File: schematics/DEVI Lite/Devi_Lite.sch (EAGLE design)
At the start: 96 parts

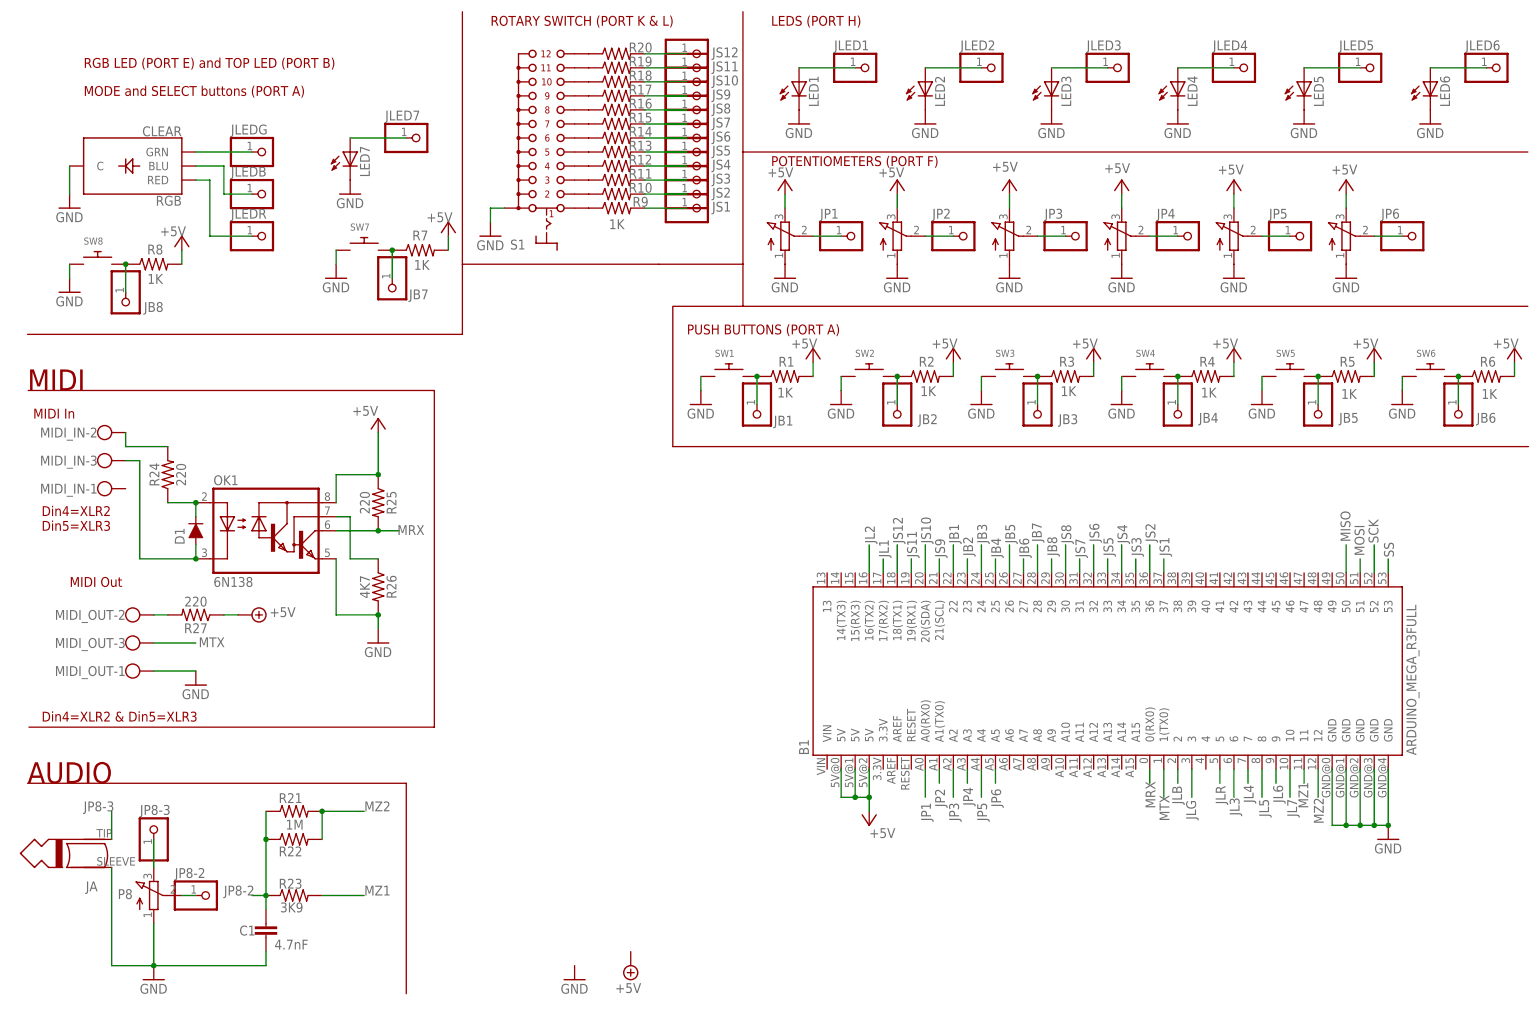
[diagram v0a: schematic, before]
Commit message: latest
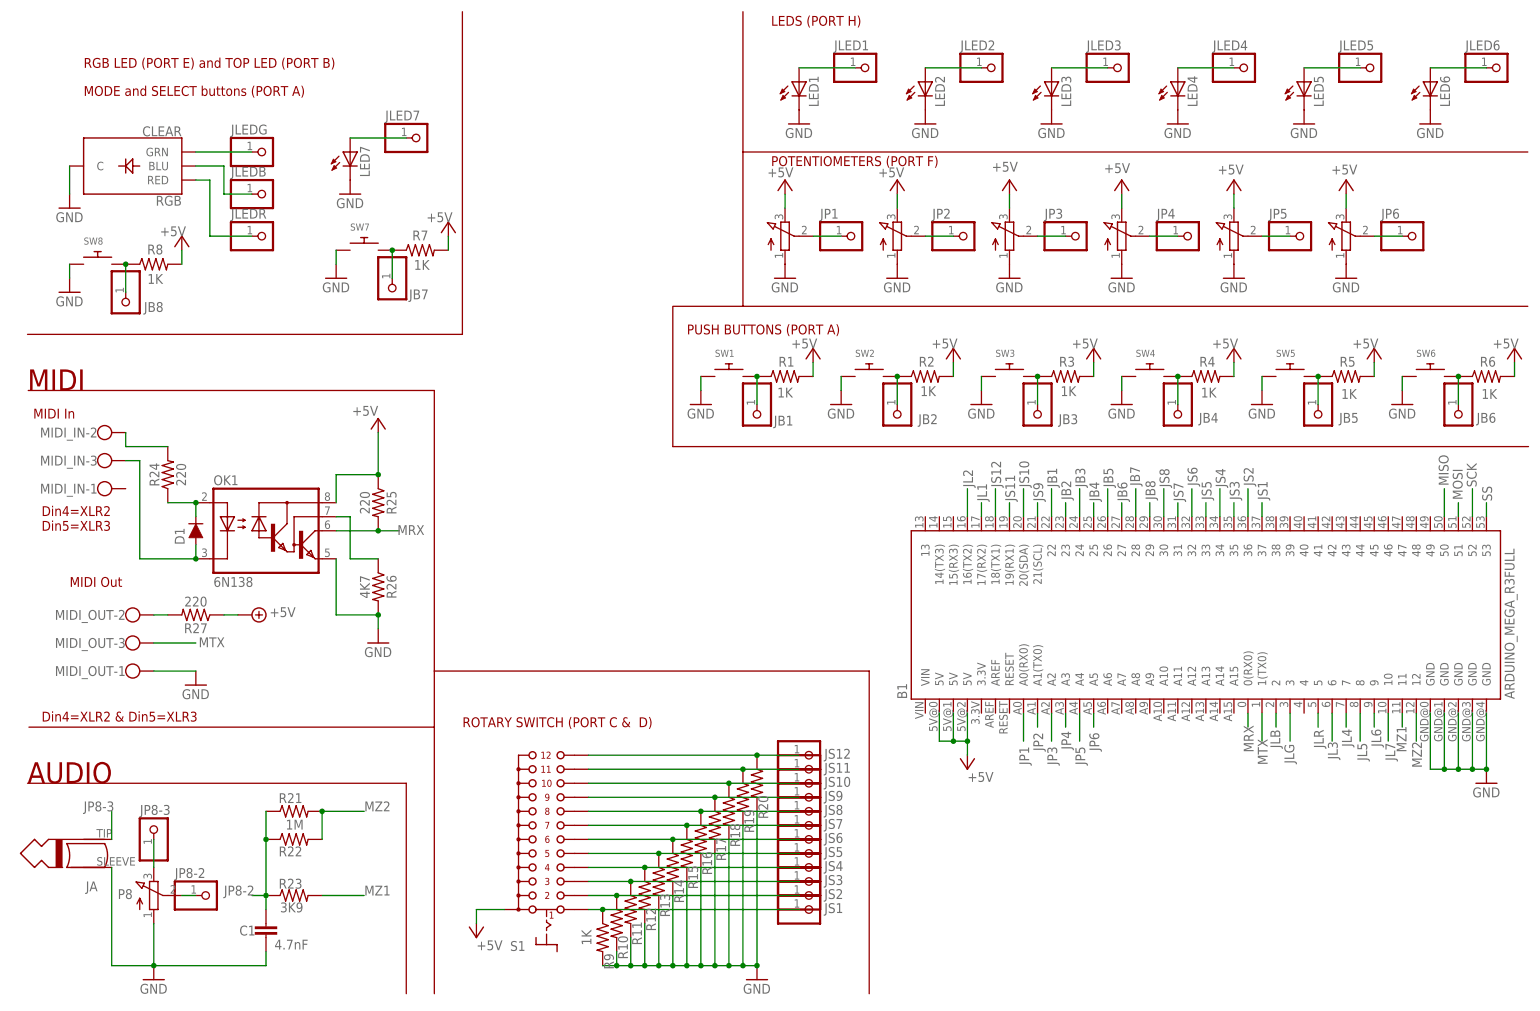
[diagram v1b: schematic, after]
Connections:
- removed net N$10: R17.1, S1.9
- removed net N$11: R18.1, S1.10
- removed net N$12: R19.1, S1.11
- removed net N$13: R20.1, S1.12
- removed net N$2: R9.1, S1.1
- removed net N$3: R10.1, S1.2
- removed net N$4: R11.1, S1.3
- removed net N$5: R12.1, S1.4
- removed net N$6: R13.1, S1.5
- removed net N$7: R14.1, S1.6
- removed net N$8: R15.1, S1.7
- removed net N$9: R16.1, S1.8
- net +5V: now also S1.A
- net GND: now also R10.2, R11.2, R12.2, R13.2, R14.2, R15.2, R16.2, R17.2, R18.2, R19.2, R20.2, R9.2; no longer S1.A
- net JS1: now also R9.1, S1.1; no longer R9.2
- net JS10: now also R18.1, S1.10; no longer R18.2
- net JS11: now also R19.1, S1.11; no longer R19.2
- net JS12: now also R20.1, S1.12; no longer R20.2
- net JS2: now also R10.1, S1.2; no longer R10.2
- net JS3: now also R11.1, S1.3; no longer R11.2
- net JS4: now also R12.1, S1.4; no longer R12.2
- net JS5: now also R13.1, S1.5; no longer R13.2
- net JS6: now also R14.1, S1.6; no longer R14.2
- net JS7: now also R15.1, S1.7; no longer R15.2
- net JS8: now also R16.1, S1.8; no longer R16.2
- net JS9: now also R17.1, S1.9; no longer R17.2
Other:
- note added: "ROTARY SWITCH (PORT C & D)"
- note removed: "ROTARY SWITCH (PORT K & L)"
- moved on the sheet: B1, JS1, JS10, JS11, JS12, JS2, JS3, JS4, JS5, JS6, JS7, JS8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
